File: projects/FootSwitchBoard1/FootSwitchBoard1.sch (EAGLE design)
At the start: 10 parts

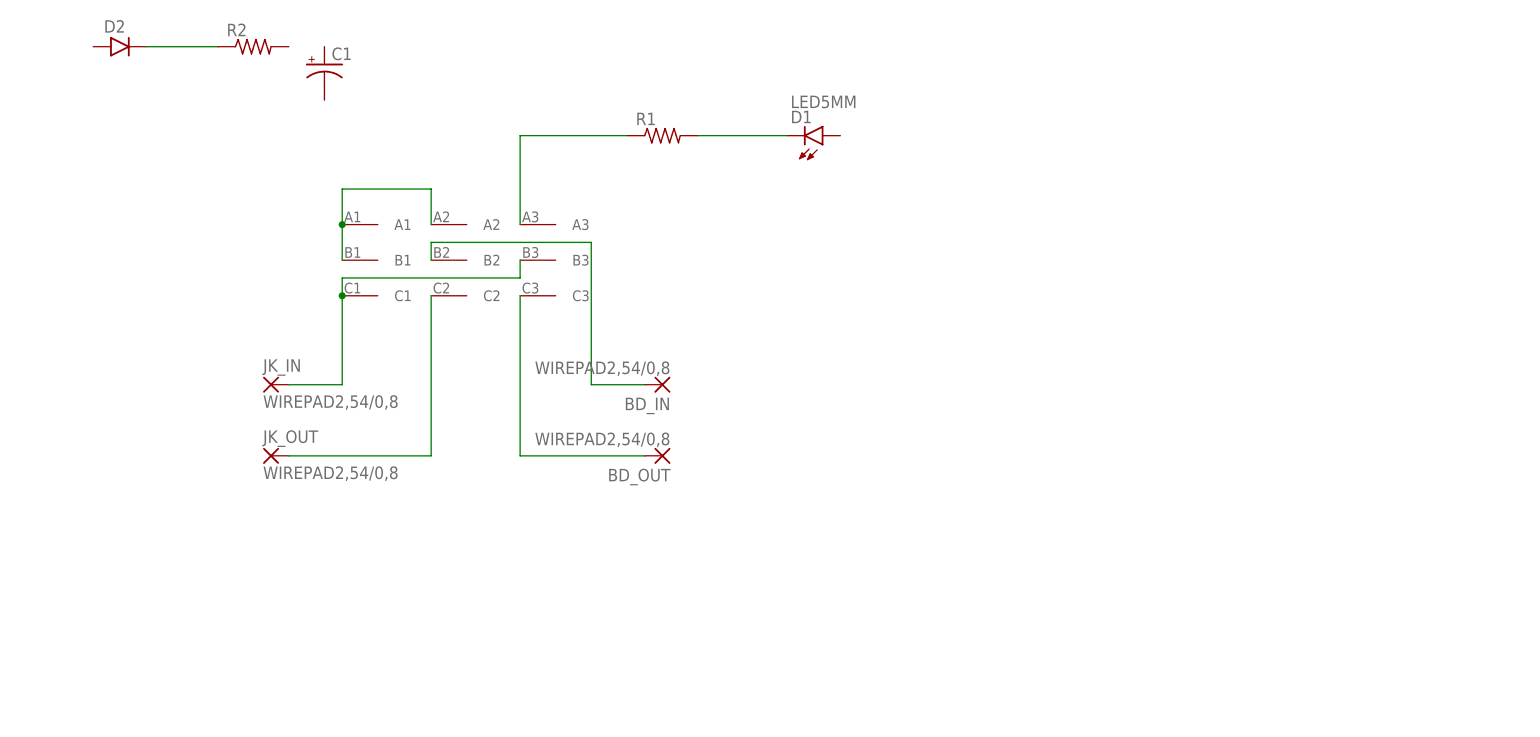
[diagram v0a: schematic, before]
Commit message: Board updates.
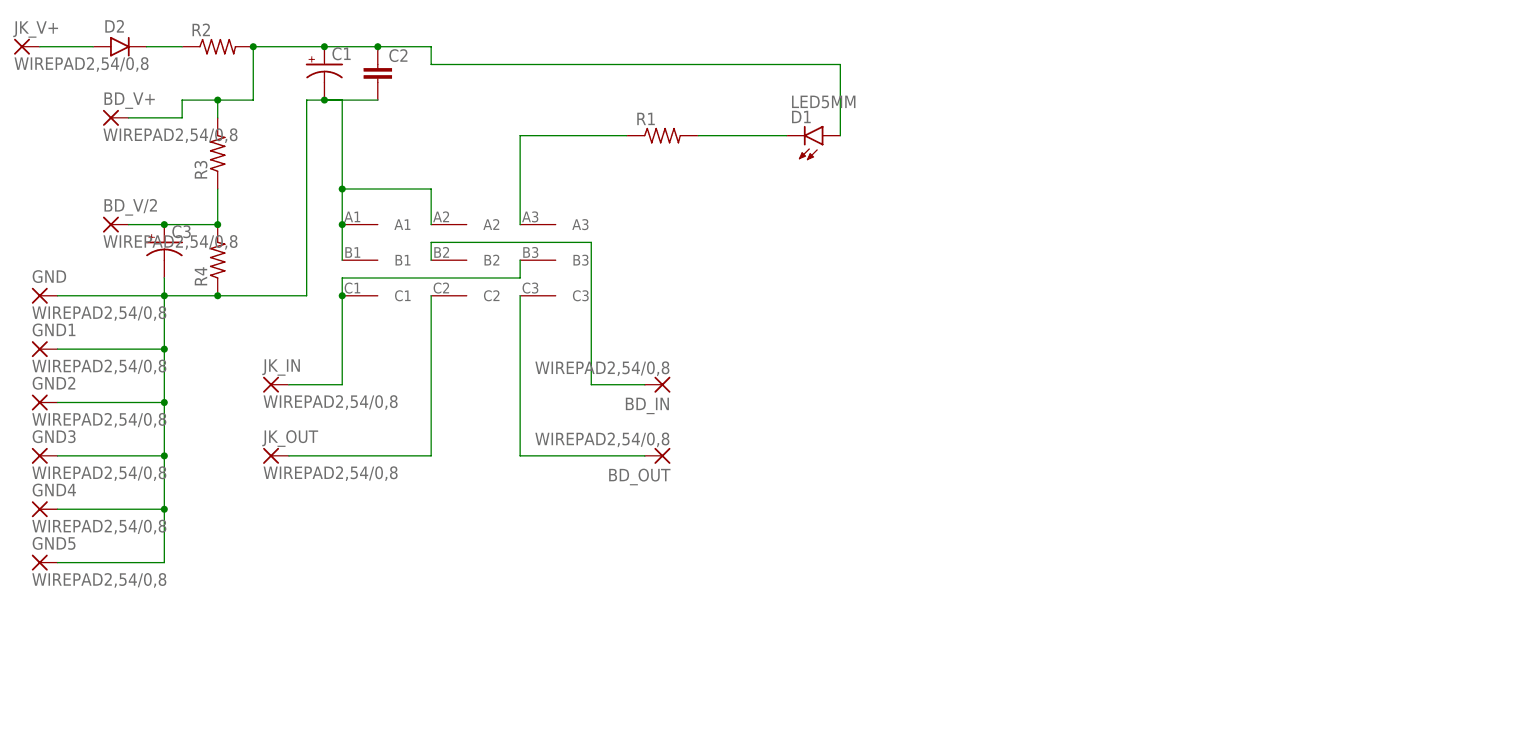
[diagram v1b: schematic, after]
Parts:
- added BD_V+, BD_V/2, GND, GND1, GND2, GND3, GND4, GND5, JK_V+: WIREPAD2,54/0,8, wirepad:WIREPAD2,54/0,8
- added C2: (no value), gm-caps-film-box:072X0352
- added C3: (no value), gm-caps-electro-pol:080
- added R3, R4: (no value), gm-resistors:6MM.4
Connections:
- new net N$10: BD_V/2.P, C3.+, R3.1, R4.2
- new net N$11: C1.-, C2.2, C3.-, GND.P, GND1.P, GND2.P, GND3.P, GND4.P, GND5.P, R4.1, U$1.A1, U$1.A2, U$1.B1
- new net N$9: BD_V+.P, C1.+, C2.1, D1.A, R2.2, R3.2
- net N$7: now also D2.A, JK_V+.P; no longer U$1.A1, U$1.A2, U$1.B1
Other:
- moved on the sheet: R2
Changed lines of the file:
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@@
 <part name="R2" library="gm-resistors" deviceset="6MM" device=".4"/>
 <part name="C1" library="gm-caps-electro-pol" deviceset="080" device=""/>
+<part name="C2" library="gm-caps-film-box" deviceset="072X035" device="2"/>
+<part name="R3" library="gm-resistors" deviceset="6MM" device=".4"/>
+<part name="R4" library="gm-resistors" deviceset="6MM" device=".4"/>
+<part name="C3" library="gm-caps-electro-pol" deviceset="080" device=""/>
+<part name="JK_V+" library="wirepad" deviceset="WIREPAD" device="2,54/0,8"/>
+<part name="GND" library="wirepad" deviceset="WIREPAD" device="2,54/0,8"/>
+<part name="BD_V/2" library="wirepad" deviceset="WIREPAD" device="2,54/0,8"/>
+<part name="BD_V+" library="wirepad" deviceset="WIREPAD" device="2,54/0,8"/>
+<part name="GND1" library="wirepad" deviceset="WIREPAD" device="2,54/0,8"/>
+<part name="GND2" library="wirepad" deviceset="WIREPAD" device="2,54/0,8"/>
+<part name="GND3" library="wirepad" deviceset="WIREPAD" device="2,54/0,8"/>
+<part name="GND4" library="wirepad" deviceset="WIREPAD" device="2,54/0,8"/>
+<part name="GND5" library="wirepad" deviceset="WIREPAD" device="2,54/0,8"/>
 </parts>
 <sheets>
@@
 <instance part="R1" gate="G$1" x="93.98" y="68.58"/>
 <instance part="D2" gate="1" x="17.78" y="81.28"/>
-<instance part="R2" gate="G$1" x="35.56" y="81.28"/>
+<instance part="R2" gate="G$1" x="30.48" y="81.28"/>
 <instance part="C1" gate="G$1" x="45.72" y="78.74"/>
+<instance part="C2" gate="G$1" x="53.34" y="76.2"/>
+<instance part="R3" gate="G$1" x="30.48" y="66.04" rot="R90"/>
+<instance part="R4" gate="G$1" x="30.48" y="50.8" rot="R90"/>
+<instance part="C3" gate="G$1" x="22.86" y="53.34"/>
+<instance part="JK_V+" gate="G$1" x="2.54" y="81.28"/>
+<instance part="GND" gate="G$1" x="5.08" y="45.72"/>
+<instance part="BD_V/2" gate="G$1" x="15.24" y="55.88"/>
+<instance part="BD_V+" gate="G$1" x="15.24" y="71.12"/>
+<instance part="GND1" gate="G$1" x="5.08" y="38.1"/>
+<instance part="GND2" gate="G$1" x="5.08" y="30.48"/>
+<instance part="GND3" gate="G$1" x="5.08" y="22.86"/>
+<instance part="GND4" gate="G$1" x="5.08" y="15.24"/>
+<instance part="GND5" gate="G$1" x="5.08" y="7.62"/>
 </instances>
 <busses>
@@
 </segment>
 </net>
-<net name="N$7" class="0">
-<segment>
+<net name="N$8" class="0">
+<segment>
+<pinref part="D2" gate="1" pin="C"/>
+<wire x1="20.32" y1="81.28" x2="25.4" y2="81.28" width="0.1524" layer="91"/>
+<pinref part="R2" gate="G$1" pin="1"/>
+</segment>
+</net>
+<net name="N$9" class="0">
+<segment>
+<pinref part="R2" gate="G$1" pin="2"/>
+<pinref part="C1" gate="G$1" pin="+"/>
+<wire x1="35.56" y1="81.28" x2="45.72" y2="81.28" width="0.1524" layer="91"/>
+<pinref part="C2" gate="G$1" pin="1"/>
+<wire x1="45.72" y1="81.28" x2="53.34" y2="81.28" width="0.1524" layer="91"/>
+<junction x="45.72" y="81.28"/>
+<wire x1="35.56" y1="81.28" x2="35.56" y2="73.66" width="0.1524" layer="91"/>
+<junction x="35.56" y="81.28"/>
+<pinref part="R3" gate="G$1" pin="2"/>
+<wire x1="35.56" y1="73.66" x2="30.48" y2="73.66" width="0.1524" layer="91"/>
+<wire x1="30.48" y1="73.66" x2="30.48" y2="71.12" width="0.1524" layer="91"/>
+<pinref part="D1" gate="G$1" pin="A"/>
+<wire x1="119.38" y1="68.58" x2="119.38" y2="78.74" width="0.1524" layer="91"/>
+<wire x1="119.38" y1="78.74" x2="60.96" y2="78.74" width="0.1524" layer="91"/>
+<wire x1="60.96" y1="78.74" x2="60.96" y2="81.28" width="0.1524" layer="91"/>
+<wire x1="60.96" y1="81.28" x2="53.34" y2="81.28" width="0.1524" layer="91"/>
+<junction x="53.34" y="81.28"/>
+<pinref part="BD_V+" gate="G$1" pin="P"/>
+<wire x1="17.78" y1="71.12" x2="25.4" y2="71.12" width="0.1524" layer="91"/>
+<wire x1="25.4" y1="71.12" x2="25.4" y2="73.66" width="0.1524" layer="91"/>
+<wire x1="25.4" y1="73.66" x2="30.48" y2="73.66" width="0.1524" layer="91"/>
+<junction x="30.48" y="73.66"/>
+</segment>
+</net>
+<net name="N$10" class="0">
+<segment>
+<pinref part="R3" gate="G$1" pin="1"/>
+<pinref part="R4" gate="G$1" pin="2"/>
+<wire x1="30.48" y1="60.96" x2="30.48" y2="55.88" width="0.1524" layer="91"/>
+<pinref part="C3" gate="G$1" pin="+"/>
+<wire x1="22.86" y1="55.88" x2="30.48" y2="55.88" width="0.1524" layer="91"/>
+<junction x="30.48" y="55.88"/>
+<pinref part="BD_V/2" gate="G$1" pin="P"/>
+<wire x1="17.78" y1="55.88" x2="22.86" y2="55.88" width="0.1524" layer="91"/>
+<junction x="22.86" y="55.88"/>
+</segment>
+</net>
+<net name="N$11" class="0">
+<segment>
+<pinref part="C3" gate="G$1" pin="-"/>
+<wire x1="22.86" y1="48.26" x2="22.86" y2="45.72" width="0.1524" layer="91"/>
+<pinref part="R4" gate="G$1" pin="1"/>
+<wire x1="22.86" y1="45.72" x2="30.48" y2="45.72" width="0.1524" layer="91"/>
+<wire x1="30.48" y1="45.72" x2="43.18" y2="45.72" width="0.1524" layer="91"/>
+<wire x1="43.18" y1="45.72" x2="43.18" y2="73.66" width="0.1524" layer="91"/>
+<junction x="30.48" y="45.72"/>
+<pinref part="C1" gate="G$1" pin="-"/>
+<wire x1="43.18" y1="73.66" x2="45.72" y2="73.66" width="0.1524" layer="91"/>
+<pinref part="C2" gate="G$1" pin="2"/>
+<wire x1="45.72" y1="73.66" x2="53.34" y2="73.66" width="0.1524" layer="91"/>
+<junction x="45.72" y="73.66"/>
 <pinref part="U$1" gate="G$1" pin="A2"/>
 <wire x1="60.96" y1="55.88" x2="60.96" y2="60.96" width="0.1524" layer="91"/>
@@
 <wire x1="48.26" y1="50.8" x2="48.26" y2="55.88" width="0.1524" layer="91"/>
 <junction x="48.26" y="55.88"/>
-</segment>
-</net>
-<net name="N$8" class="0">
-<segment>
-<pinref part="D2" gate="1" pin="C"/>
-<wire x1="20.32" y1="81.28" x2="30.48" y2="81.28" width="0.1524" layer="91"/>
-<pinref part="R2" gate="G$1" pin="1"/>
-</segment>
-</net>
+<wire x1="45.72" y1="73.66" x2="48.26" y2="73.66" width="0.1524" layer="91"/>
+<wire x1="48.26" y1="73.66" x2="48.26" y2="60.96" width="0.1524" layer="91"/>
+<junction x="48.26" y="60.96"/>
+<pinref part="GND" gate="G$1" pin="P"/>
+<wire x1="7.62" y1="45.72" x2="22.86" y2="45.72" width="0.1524" layer="91"/>
+<junction x="22.86" y="45.72"/>
+<pinref part="GND1" gate="G$1" pin="P"/>
+<wire x1="7.62" y1="38.1" x2="22.86" y2="38.1" width="0.1524" layer="91"/>
+<wire x1="22.86" y1="38.1" x2="22.86" y2="45.72" width="0.1524" layer="91"/>
+<pinref part="GND2" gate="G$1" pin="P"/>
+<wire x1="7.62" y1="30.48" x2="22.86" y2="30.48" width="0.1524" layer="91"/>
+<wire x1="22.86" y1="30.48" x2="22.86" y2="38.1" width="0.1524" layer="91"/>
+<junction x="22.86" y="38.1"/>
+<pinref part="GND3" gate="G$1" pin="P"/>
+<wire x1="7.62" y1="22.86" x2="22.86" y2="22.86" width="0.1524" layer="91"/>
+<wire x1="22.86" y1="22.86" x2="22.86" y2="30.48" width="0.1524" layer="91"/>
+<junction x="22.86" y="30.48"/>
+<pinref part="GND4" gate="G$1" pin="P"/>
+<wire x1="7.62" y1="15.24" x2="22.86" y2="15.24" width="0.1524" layer="91"/>
+<wire x1="22.86" y1="15.24" x2="22.86" y2="22.86" width="0.1524" layer="91"/>
+<junction x="22.86" y="22.86"/>
+<pinref part="GND5" gate="G$1" pin="P"/>
+<wire x1="7.62" y1="7.62" x2="22.86" y2="7.62" width="0.1524" layer="91"/>
+<wire x1="22.86" y1="7.62" x2="22.86" y2="15.24" width="0.1524" layer="91"/>
+<junction x="22.86" y="15.24"/>
+</segment>
+</net>
+<net name="N$7" class="0">
+<segment>
+<pinref part="JK_V+" gate="G$1" pin="P"/>
+<pinref part="D2" gate="1" pin="A"/>
+<wire x1="5.08" y1="81.28" x2="12.7" y2="81.28" width="0.1524" layer="91"/>
+</segment>
+</net>

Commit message: Board layout in progress.
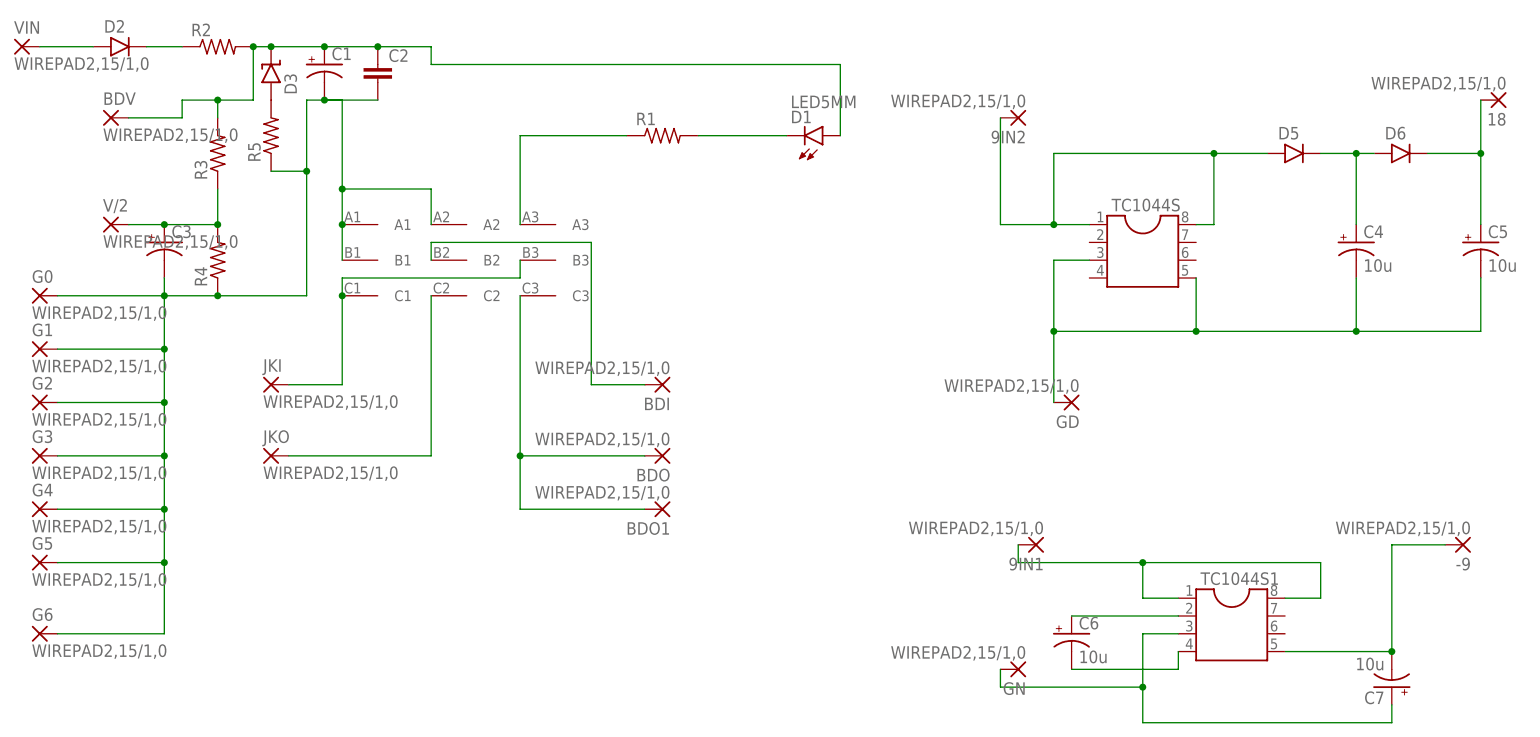
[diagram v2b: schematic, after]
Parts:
- removed BD_IN, BD_OUT, BD_V+, BD_V/2, GND, GND1, GND2, GND3, GND4, GND5, JK_IN, JK_OUT, JK_V+: WIREPAD2,54/0,8, wirepad:WIREPAD2,54/0,8
- added -9, 18, 9IN1, 9IN2, BDI, BDO, BDO1, BDV, G0, G1, G2, G3, G4, G5, G6, GD, GN, JKI, JKO, V/2, VIN: WIREPAD2,15/1,0, wirepad:WIREPAD2,15/1,0
- added C4, C5, C6, C7: 10u, gm-caps-electro-pol:050
- added D3: (no value), gm-diodes:1N9ZENER
- added D5, D6: (no value), gm-diodes:1N400X.3
- added R5: (no value), gm-resistors:10MM
- added TC1044S, TC1044S1: (no value), ic-package:DIL8S
- R1, R2, R3, R4: device gm-resistors:6MM.4 -> gm-resistors:6MM.3
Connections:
- new net -9GND: C7.+, GN.P, TC1044S1.3
- new net 18VGND: C4.-, C5.-, GD.P, TC1044S.3, TC1044S.5
- new net N$12: D3.A, R5.2
- new net N$13: 9IN2.P, D5.A, TC1044S.1, TC1044S.8
- new net N$14: C4.+, D5.C, D6.A
- new net N$15: 18.P, C5.+, D6.C
- new net N$16: 9IN1.P, TC1044S1.1, TC1044S1.8
- new net N$17: -9.P, C7.-, TC1044S1.5
- new net N$20: C6.+, TC1044S1.2
- new net N$21: C6.-, TC1044S1.4
- net N$1: now also JKI.P; no longer JK_IN.P
- net N$10: now also V/2.P; no longer BD_V/2.P
- net N$11: now also G0.P, G1.P, G2.P, G3.P, G4.P, G5.P, G6.P, R5.1; no longer GND.P, GND1.P, GND2.P, GND3.P, GND4.P, GND5.P
- net N$2: now also JKO.P; no longer JK_OUT.P
- net N$3: now also BDO.P, BDO1.P; no longer BD_OUT.P
- net N$4: now also BDI.P; no longer BD_IN.P
- net N$7: now also VIN.P; no longer JK_V+.P
- net N$9: now also BDV.P, D3.C; no longer BD_V+.P
